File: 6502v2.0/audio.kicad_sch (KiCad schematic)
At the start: 22 parts, among them J16 AudioPlug3, U13 PSG_AY-3-8910, U15 PSG_AY-3-8910

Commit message: working on pcb
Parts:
- C16, C18, C19, C20: footprint (none) -> Capacitor_THT:C_Disc_D5.1mm_W3.2mm_P5.00mm
- R14, R15, R16, R17, R18, R19, R20, R21, R22, R23, R24, R25: footprint (none) -> Resistor_THT:R_Axial_DIN0204_L3.6mm_D1.6mm_P7.62mm_Horizontal
- U13, U15: footprint (none) -> Package_DIP:DIP-40_W15.24mm_Socket
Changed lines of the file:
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@@
       (effects (font (size 1.27 1.27)) (justify left))
     )
-    (property "Footprint" "" (at 113.792 45.72 90)
+    (property "Footprint" "Resistor_THT:R_Axial_DIN0204_L3.6mm_D1.6mm_P7.62mm_Horizontal" (at 113.792 45.72 90)
       (effects (font (size 1.27 1.27)) hide)
     )
@@
       (effects (font (size 1.27 1.27)) (justify left))
     )
-    (property "Footprint" "" (at 113.792 102.87 90)
+    (property "Footprint" "Resistor_THT:R_Axial_DIN0204_L3.6mm_D1.6mm_P7.62mm_Horizontal" (at 113.792 102.87 90)
       (effects (font (size 1.27 1.27)) hide)
     )
@@
       (effects (font (size 1.27 1.27)) (justify right))
     )
-    (property "Footprint" "" (at 85.598 114.3 90)
+    (property "Footprint" "Resistor_THT:R_Axial_DIN0204_L3.6mm_D1.6mm_P7.62mm_Horizontal" (at 85.598 114.3 90)
       (effects (font (size 1.27 1.27)) hide)
     )
@@
       (effects (font (size 1.27 1.27)) (justify right))
     )
-    (property "Footprint" "" (at 184.658 69.85 90)
+    (property "Footprint" "Resistor_THT:R_Axial_DIN0204_L3.6mm_D1.6mm_P7.62mm_Horizontal" (at 184.658 69.85 90)
       (effects (font (size 1.27 1.27)) hide)
     )
@@
       (effects (font (size 1.27 1.27)) (justify left))
     )
-    (property "Footprint" "" (at 189.992 77.47 90)
+    (property "Footprint" "Resistor_THT:R_Axial_DIN0204_L3.6mm_D1.6mm_P7.62mm_Horizontal" (at 189.992 77.47 90)
       (effects (font (size 1.27 1.27)) hide)
     )
@@
       (effects (font (size 1.27 1.27)) (justify left))
     )
-    (property "Footprint" "" (at 82.042 121.92 90)
+    (property "Footprint" "Resistor_THT:R_Axial_DIN0204_L3.6mm_D1.6mm_P7.62mm_Horizontal" (at 82.042 121.92 90)
       (effects (font (size 1.27 1.27)) hide)
     )
@@
       (effects (font (size 1.27 1.27)) (justify right))
     )
-    (property "Footprint" "" (at 94.488 114.3 90)
+    (property "Footprint" "Resistor_THT:R_Axial_DIN0204_L3.6mm_D1.6mm_P7.62mm_Horizontal" (at 94.488 114.3 90)
       (effects (font (size 1.27 1.27)) hide)
     )
@@
       (effects (font (size 1.27 1.27)) (justify left))
     )
-    (property "Footprint" "" (at 16.002 36.83 90)
+    (property "Footprint" "Resistor_THT:R_Axial_DIN0204_L3.6mm_D1.6mm_P7.62mm_Horizontal" (at 16.002 36.83 90)
       (effects (font (size 1.27 1.27)) hide)
     )
@@
       (effects (font (size 1.27 1.27)) (justify left))
     )
-    (property "Footprint" "" (at 210.5152 92.71 0)
+    (property "Footprint" "Capacitor_THT:C_Disc_D5.1mm_W3.2mm_P5.00mm" (at 210.5152 92.71 0)
       (effects (font (size 1.27 1.27)) hide)
     )
@@
       (effects (font (size 1.27 1.27)) (justify left))
     )
-    (property "Footprint" "" (at 26.162 95.25 90)
+    (property "Footprint" "Resistor_THT:R_Axial_DIN0204_L3.6mm_D1.6mm_P7.62mm_Horizontal" (at 26.162 95.25 90)
       (effects (font (size 1.27 1.27)) hide)
     )
@@
       (effects (font (size 1.27 1.27)))
     )
-    (property "Footprint" "" (at 217.17 72.6948 0)
+    (property "Footprint" "Capacitor_THT:C_Disc_D5.1mm_W3.2mm_P5.00mm" (at 217.17 72.6948 0)
       (effects (font (size 1.27 1.27)) hide)
     )
@@
       (effects (font (size 1.27 1.27)) (justify right))
     )
-    (property "Footprint" "" (at 193.548 69.85 90)
+    (property "Footprint" "Resistor_THT:R_Axial_DIN0204_L3.6mm_D1.6mm_P7.62mm_Horizontal" (at 193.548 69.85 90)
       (effects (font (size 1.27 1.27)) hide)
     )
@@
       (effects (font (size 1.27 1.27)) (justify left))
     )
-    (property "Footprint" "" (at 102.5652 137.16 0)
+    (property "Footprint" "Capacitor_THT:C_Disc_D5.1mm_W3.2mm_P5.00mm" (at 102.5652 137.16 0)
       (effects (font (size 1.27 1.27)) hide)
     )
@@
       (effects (font (size 1.27 1.27)))
     )
-    (property "Footprint" "" (at 109.22 117.1448 0)
+    (property "Footprint" "Capacitor_THT:C_Disc_D5.1mm_W3.2mm_P5.00mm" (at 109.22 117.1448 0)
       (effects (font (size 1.27 1.27)) hide)
     )
@@
       (effects (font (size 1.27 1.27)) (justify right))
     )
-    (property "Footprint" "" (at 202.438 69.85 90)
+    (property "Footprint" "Resistor_THT:R_Axial_DIN0204_L3.6mm_D1.6mm_P7.62mm_Horizontal" (at 202.438 69.85 90)
       (effects (font (size 1.27 1.27)) hide)
     )
@@
       (effects (font (size 1.27 1.27)) (justify left))
     )
-    (property "Footprint" "" (at 58.42 34.29 0)
+    (property "Footprint" "Package_DIP:DIP-40_W15.24mm_Socket" (at 58.42 34.29 0)
       (effects (font (size 1.27 1.27)) hide)
     )
@@
       (effects (font (size 1.27 1.27)) (justify left))
     )
-    (property "Footprint" "" (at 142.24 50.8 0)
+    (property "Footprint" "Package_DIP:DIP-40_W15.24mm_Socket" (at 142.24 50.8 0)
       (effects (font (size 1.27 1.27)) hide)
     )
@@
       (effects (font (size 1.27 1.27)) (justify right))
     )
-    (property "Footprint" "" (at 76.708 114.3 90)
-      (effects (font (size 1.27 1.27)) hide)
-    )
+    (property "Footprint" "Resistor_THT:R_Axial_DIN0204_L3.6mm_D1.6mm_P7.62mm_Horizontal" (at 76.708 114.3 90)
+      (effects (font (size 1.27 1.27)) hide)
+    )

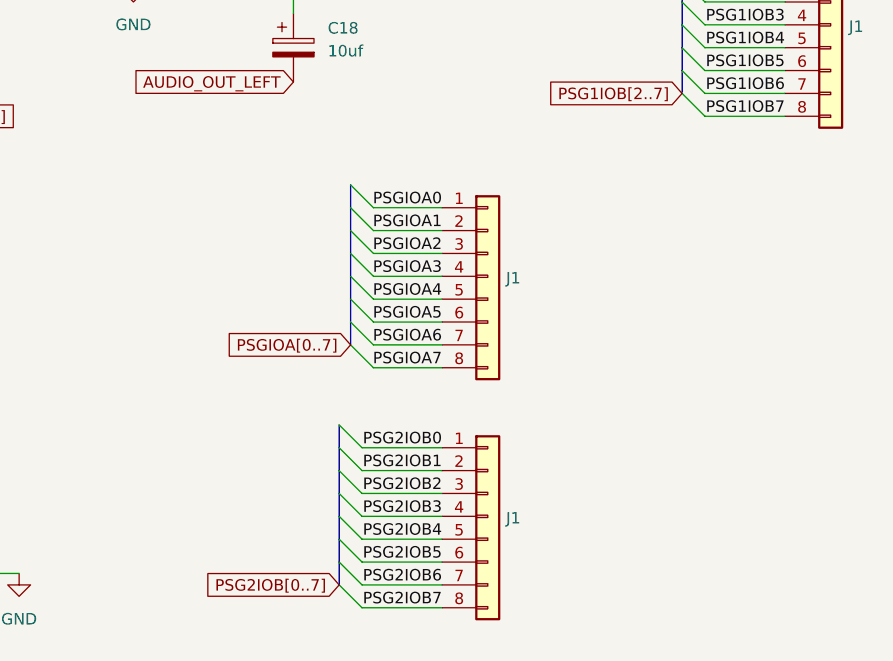
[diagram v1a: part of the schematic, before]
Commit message: worked on video card
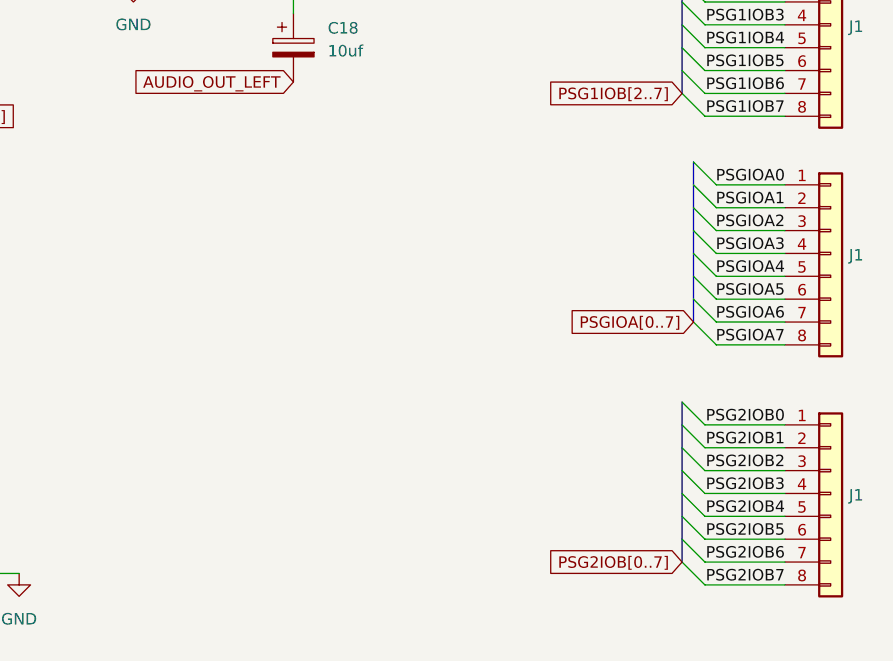
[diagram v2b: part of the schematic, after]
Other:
- moved on the sheet: J1
